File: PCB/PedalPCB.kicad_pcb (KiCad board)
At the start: 2 copper layers, 45.5 x 73.5 mm, 13 parts, among them J2 Break, J3 Throttle, J4 SystemInput, J5 Conn_01x04_Socket

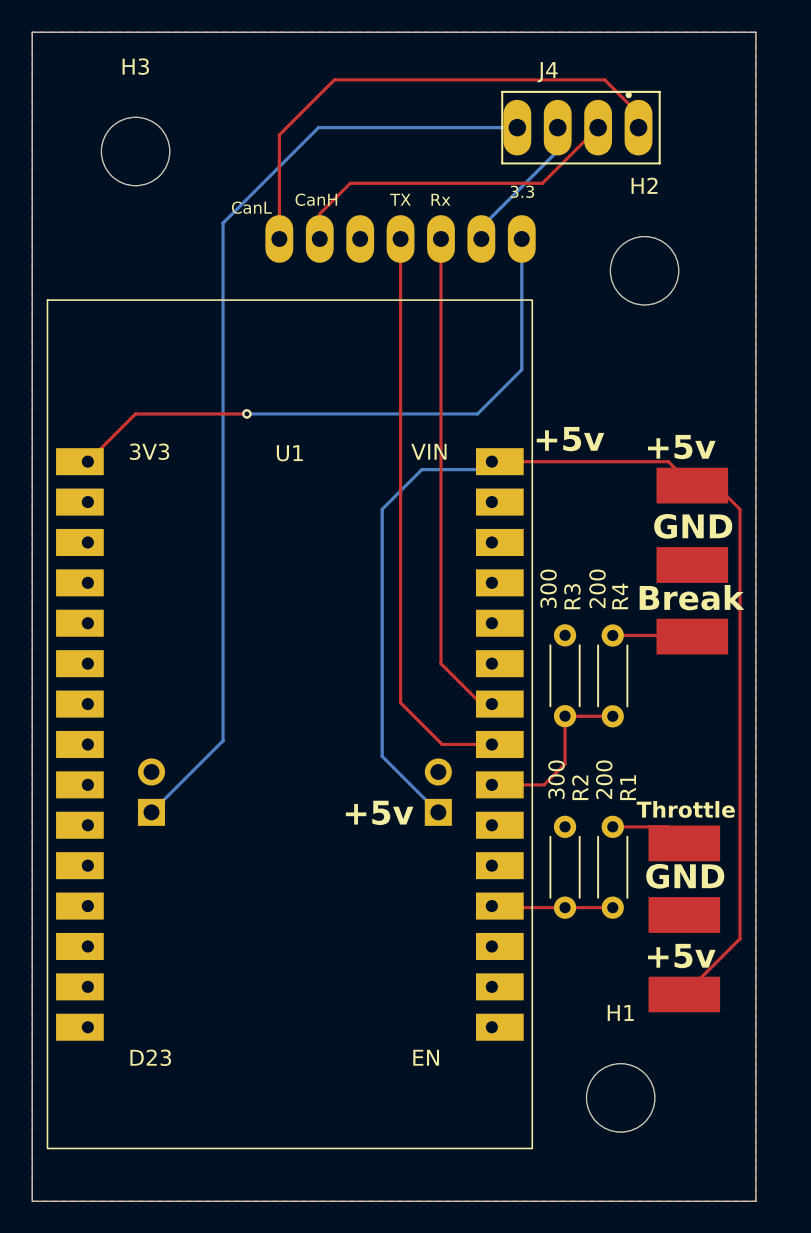
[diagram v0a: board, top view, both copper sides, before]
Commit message: Update PCB to purchased version
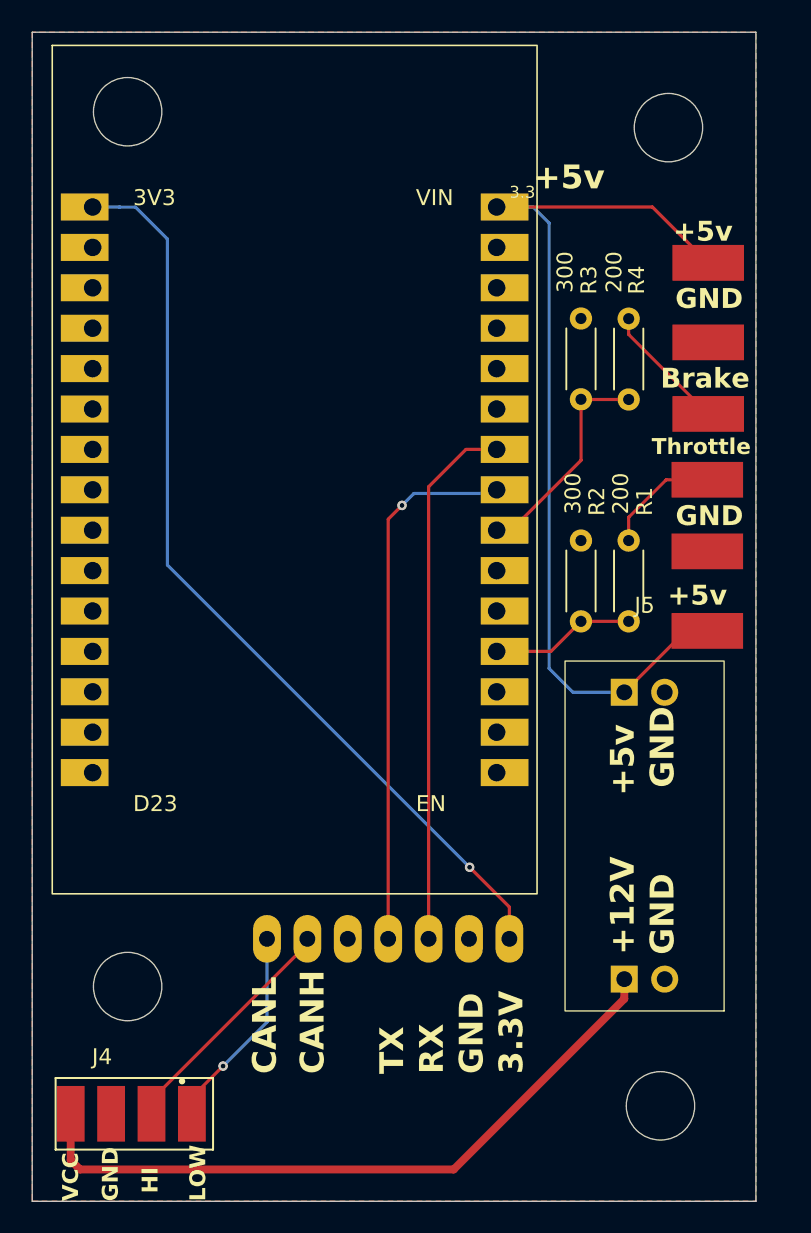
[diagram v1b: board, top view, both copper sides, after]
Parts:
- added H1: MountingHole, MountingHole:MountingHole_4.3mm_M4, F.Cu at (111.0, 109.0)
- J5: moved to F.Cu
- moved J4 68.1 mm to (111.4, 117.0)
- moved U2 44.0 mm to (135.0, 106.0)
- moved J3 22.9 mm to (147.4, 70.6)
- moved R3 19.9 mm to (139.5, 72.1)
- moved R4 19.9 mm to (142.5, 67.0)
- moved R1 18.0 mm to (142.5, 81.0)
- moved R2 18.0 mm to (139.5, 86.0)
- moved U1 16.0 mm to (121.5, 60.0)
- moved J2 14.0 mm to (147.5, 79.5)
- moved J5 13.8 mm to (143.5, 85.5), turned to 0 degrees
- moved H2 9.12 mm to (145.0, 55.0)
- moved H1 2.55 mm to (144.5, 116.5)
- moved H3 2.55 mm to (111.0, 54.0)
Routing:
- net +3.3V: track 37.9 -> 58.4 mm
- net /CanL: track 32.3 -> 13.0 mm, vias 0 -> 1
- net +5V: track 77.4 -> 58.6 mm
- net +12V: track 59.9 -> 43.6 mm
- net GND: track 8.99 -> 0.00 mm
- net /CanH: track 21.3 -> 15.1 mm
- net Net-(J2-Pin_1): track 5.03 -> 8.06 mm
- net /Break: track 11.1 -> 14.0 mm
- net Net-(J3-Pin_1): track 4.93 -> 7.38 mm
- net /CanRX: track 31.3 -> 33.7 mm
- net /CanTX: track 36.1 -> 34.0 mm, vias 0 -> 1
- net /Throttle: track 7.54 -> 9.08 mm
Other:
- board text added: "+12V"
- board text added: "3.3V"
- board text added: "Brake"
- board text added: "CANH"
- board text added: "CANL"
- board text added: "HI"
- board text added: "LOW"
- board text added: "RX"
- board text added: "VCC"
- board text removed: "12+"
- board text removed: "Break"
- board text removed: "CanH"
- board text removed: "CanL"
- board text removed: "Rx"
